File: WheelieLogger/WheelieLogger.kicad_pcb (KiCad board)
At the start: 2 copper layers, 28.8 x 22 mm, 30 parts, among them J1 USB_C_Plug_USB2.0, J2 Conn_Power, J3 TC2030-IDC-NL, SW1 SW_RESET, U1 GD25Q32CNIGR, U2 MCP1700-3302E_SOT23, U3 ATSAMD21E18A, U4 MPU-6050

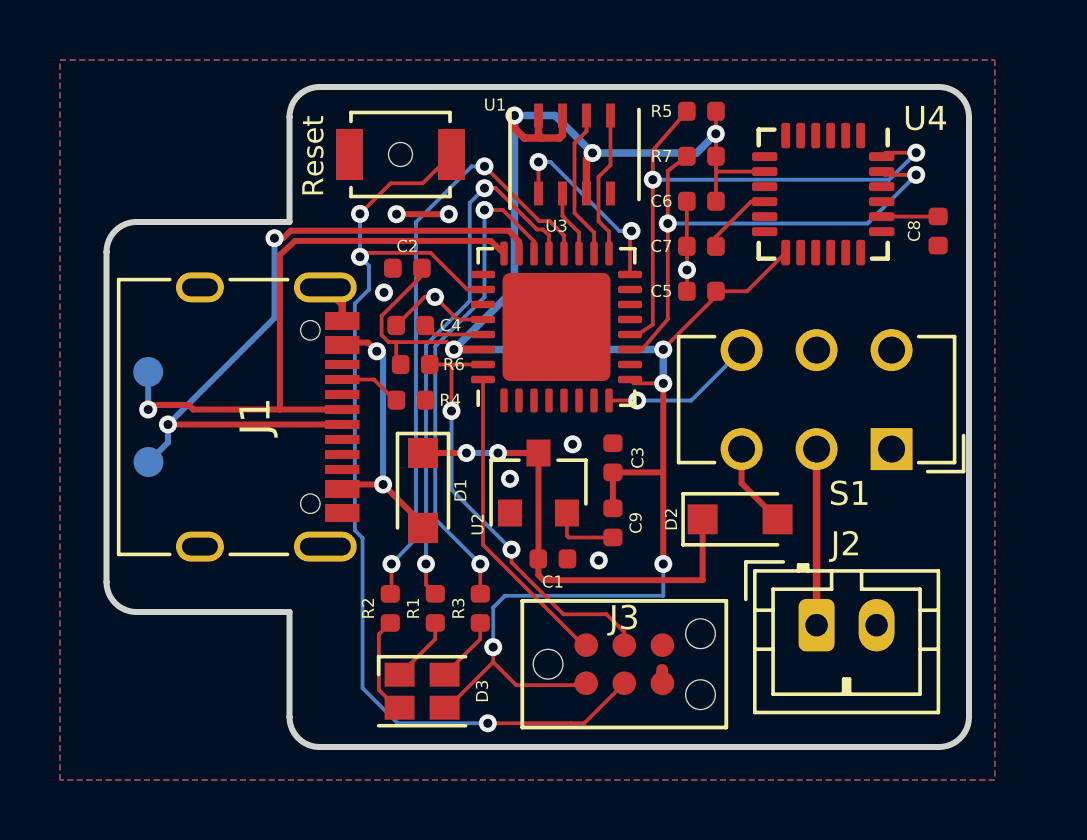
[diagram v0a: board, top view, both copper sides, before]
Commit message: Updated to version 2
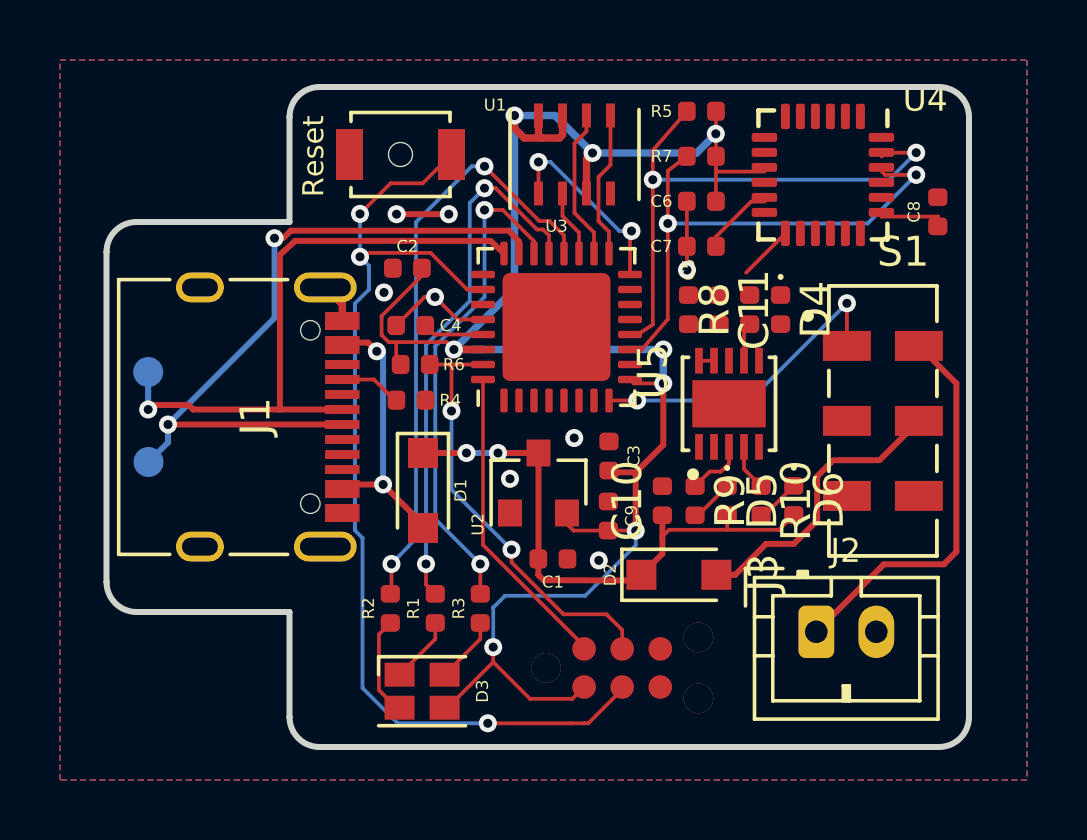
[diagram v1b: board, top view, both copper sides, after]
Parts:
- added C10: 1uF, Capacitor_SMD:C_0402_1005Metric, F.Cu at (150.1, 91.7)
- added C11: 1uF, Capacitor_SMD:C_0402_1005Metric, F.Cu at (152.0, 85.3)
- added D4: Red, LED_SMD:LED_0402_1005Metric, F.Cu at (154.0, 85.3)
- added D5: Yellow, LED_SMD:LED_0402_1005Metric, F.Cu at (152.2, 91.7)
- added D6: Green, LED_SMD:LED_0402_1005Metric, F.Cu at (154.5, 91.7)
- added R10: 1.5kR, Resistor_SMD:R_0402_1005Metric, F.Cu at (153.4, 91.7)
- added R8: 1.5kR, Resistor_SMD:R_0402_1005Metric, F.Cu at (153.0, 85.3)
- added R9: 1.5kR, Resistor_SMD:R_0402_1005Metric, F.Cu at (151.2, 91.7)
- added U5: MCP73833-AMI_UN, Footprints:SON50P300X300X100-11N, F.Cu at (152.3, 88.5)
- J3: footprint TC2030:TAG_TC2030-IDC-NL -> Footprints:Tag-Connect_TC2030-IDC-NL
- S1: footprint Button_Switch_THT:SW_CuK_JS202011CQN_DPDT_Straight -> Footprints:SW_JS202011JCQN
- moved D2 2.75 mm to (150.6, 94.2)
- moved J3 1.54 mm to (147.5, 97.9)
- moved S1 0.98 mm to (157.4, 89.0), turned to 0 degrees
- moved C5 0.75 mm to (150.9, 85.3), turned to -90 degrees
- moved C8 0.64 mm to (159.3, 82.1)
- moved U4 0.64 mm to (155.4, 80.8)
- moved C9 0.27 mm to (148.3, 92.2)
- moved J2 0.22 mm to (155.2, 96.1)
- moved C3 0.14 mm to (148.3, 90.2)
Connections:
- C9 pad 1: +3V3 -> GND
- C9 pad 2: Net-(C9-Pad2) -> +3V3
- S1 pad 1: Net-(S1-Pad1) -> /GPIO3
- S1 pad 2: /PWR_SW -> GND
- S1 pad 3: VIN -> Net-(S1-Pad3)
- S1 pad 5: GND -> /PWR_SW
- S1 pad 6: /GPIO3 -> VIN
- U2 pad 2: Net-(C9-Pad2) -> +3V3
- U4 pad 9: Net-(U4-Pad9) -> +3V3
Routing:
- net VIN: track 2.84 -> 10.2 mm
- net /PWR_SW: track 5.87 -> 13.2 mm
- net /GPIO3: track 5.12 -> 10.7 mm, vias 1 -> 2
- net +3V3: track 71.8 -> 67.1 mm
- net +5V: track 15.5 -> 18.9 mm
- net Net-(C9-Pad2): track 2.31 -> 0.00 mm
- net Net-(R9-Pad1): track 0.00 -> 2.00 mm
- net Net-(C8-Pad2): track 1.89 -> 0.00 mm
- net Net-(R10-Pad1): track 0.00 -> 1.55 mm
- net Net-(D6-Pad1): track 0.00 -> 1.50 mm
- net Net-(D5-Pad1): track 0.00 -> 1.47 mm
- net Net-(R8-Pad1): track 0.00 -> 1.31 mm
- net GND: track 10.2 -> 10.8 mm
